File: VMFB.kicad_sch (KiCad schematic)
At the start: 137 parts, among them J1 Screw_Terminal_01x02, J10 Conn_01x03_Pin, J11 Conn_01x08_Pin, J12 Conn_01x06_Pin, J13 Conn_01x03_Pin, J14 Conn_01x03_Pin, J15 Conn_01x03_Pin, J16 Conn_01x03_Pin, J17 Conn_01x03_Pin, J18 Conn_01x03_Pin, J19 Conn_01x02_Pin, J2 USB_A_Stacked, J20 Conn_01x03_Pin, J21 Conn_01x02_Pin, J3 USB_B, J4 Barrel_Jack_Switch, J5 Conn_01x02_Pin, J6 Conn_01x03_Pin, J7 Conn_01x02_Pin, J8 Conn_01x03_Pin, J9 Conn_01x03_Pin, Q1 BC547B, Q2 TIP41C, Q3 BC547B, Q4 BC547B, Q5 BD139, Q6 BC547B, Q7 BC547B, Q8 BC547, U1 NE555P, U2 NE555P, U3 LM358, U4 NE555P, U5 NE555P

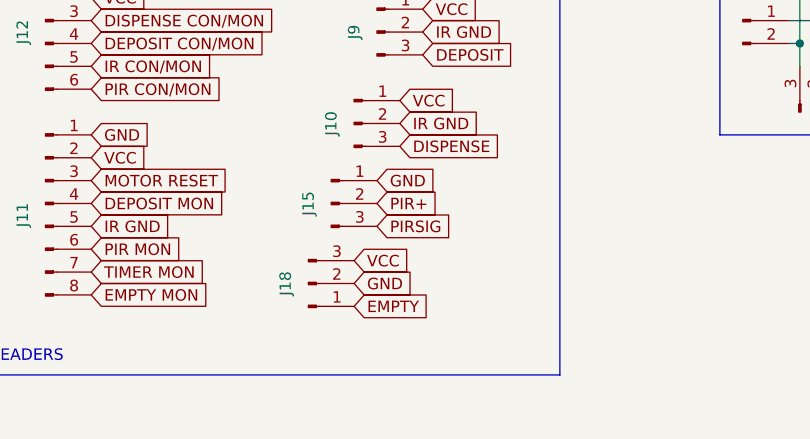
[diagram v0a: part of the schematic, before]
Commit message: schemati and pcb tweaking
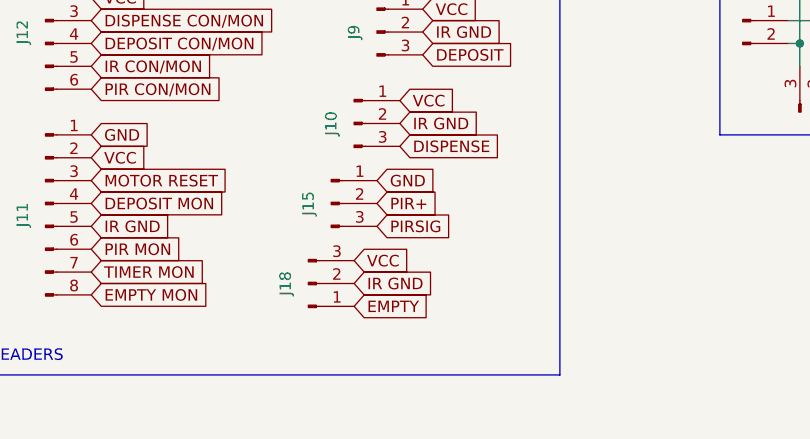
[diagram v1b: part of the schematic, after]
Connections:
- net GND: no longer J18.2 (Pin_2)
- net IR GND: now also J18.2 (Pin_2)
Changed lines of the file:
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@@
     )
   )
-  (global_label "GND" (shape input) (at 137.16 181.61 0) (fields_autoplaced)
+  (global_label "IR GND" (shape input) (at 137.16 181.61 0) (fields_autoplaced)
     (effects (font (size 1.27 1.27)) (justify left))
-    (property "Intersheetrefs" "${INTERSHEET_REFS}" (at 143.9363 181.61 0) (show_name)
+    (property "Intersheetrefs" "${INTERSHEET_REFS}" (at 146.7787 181.61 0) (show_name)
       (effects (font (size 1.27 1.27)) (justify left) hide)
     )
